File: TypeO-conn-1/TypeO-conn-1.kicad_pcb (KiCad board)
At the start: 2 copper layers, 5 parts, among them J1 USB_C_Receptacle_USB2.0, J2 , SW1 SW_DIP_x01

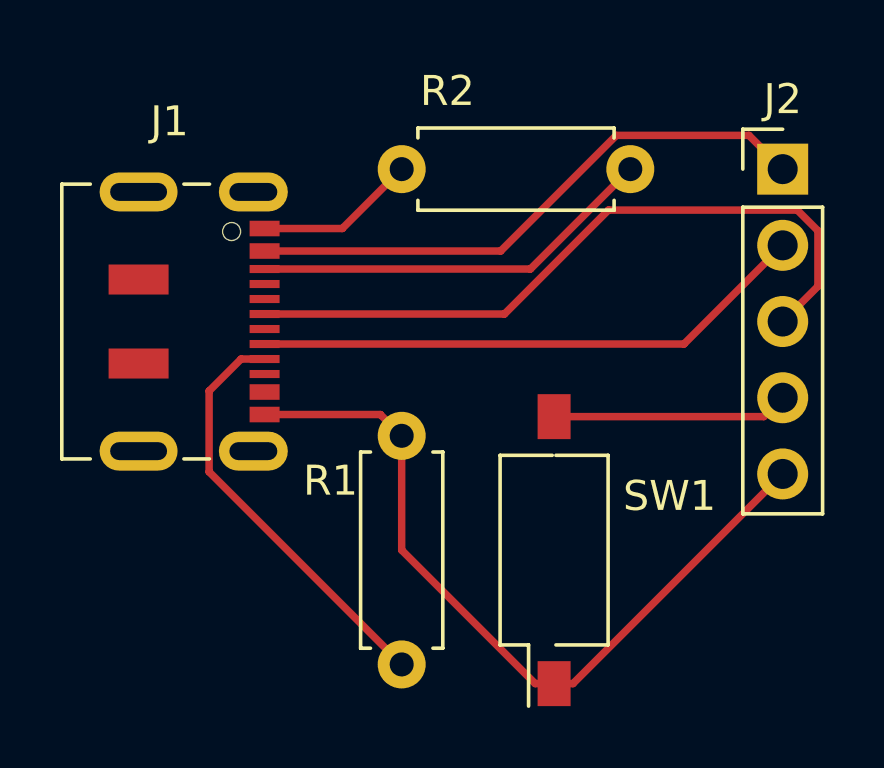
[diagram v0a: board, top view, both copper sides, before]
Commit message: Update PCB
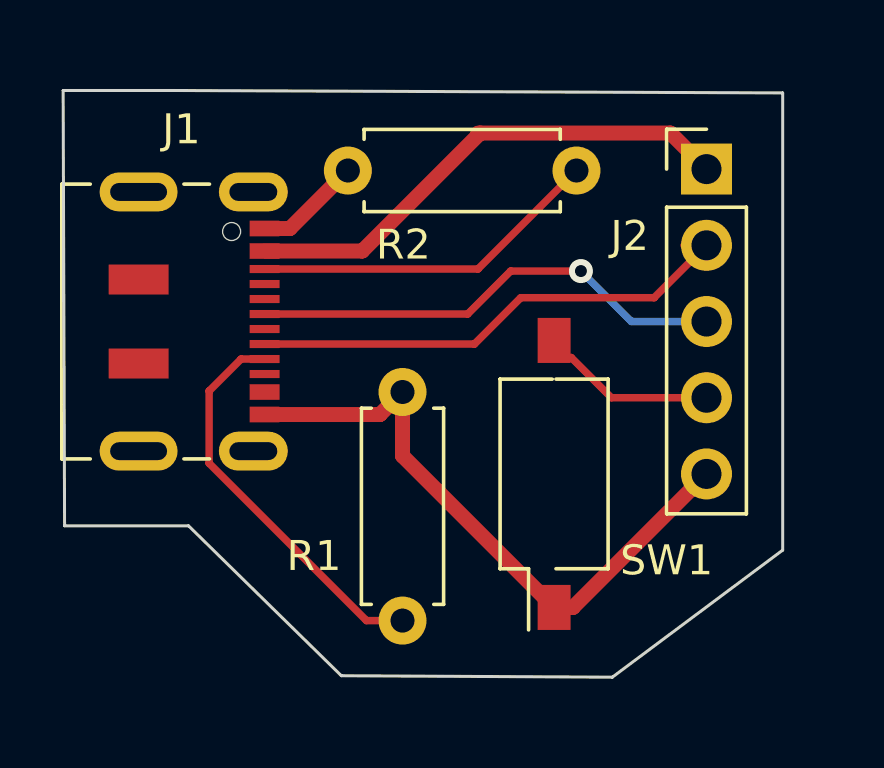
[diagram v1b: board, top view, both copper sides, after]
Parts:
- moved J2 2.54 mm to (124.5, 76.2)
- moved SW1 2.54 mm to (119.4, 86.4)
- moved R2 1.79 mm to (112.5, 76.2)
- moved R1 1.46 mm to (114.3, 83.6)
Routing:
- net Net-(J1-PadA6): track 23.7 -> 16.0 mm, vias 0 -> 1
- net Net-(J1-PadA1): track 31.5 -> 24.7 mm
- net Net-(J1-PadA4): track 19.3 -> 16.9 mm
- net Net-(SW1-Pad2): track 7.88 -> 5.64 mm
- net Net-(J1-PadA5): track 13.6 -> 11.8 mm
- net Net-(J1-PadA7): track 18.6 -> 16.8 mm
- net Net-(J1-PadB5): track 14.1 -> 13.3 mm
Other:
- board outline added: 24 x 19.6 mm
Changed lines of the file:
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@@
     (property "Sheetname" "")
     (attr smd)
-    (fp_text reference "J1" (at -6.670499 0.12134 180) (layer "F.SilkS")
+    (fp_text reference "J1" (at -6.404035 -0.274964 180) (layer "F.SilkS")
       (effects (font (size 1 1) (thickness 0.15)))
     )
@@
   )
   (footprint "Resistor_THT:R_Axial_DIN0207_L6.3mm_D2.5mm_P7.62mm_Horizontal" (layer "F.Cu")
-    (at 114.3 76.2)
+    (at 112.505976 76.246718)
     (descr "Resistor, Axial_DIN0207 series, Axial, Horizontal, pin pitch=7.62mm, 0.25W = 1/4W, length*diameter=6.3*2.5mm^2, http://cdn-reichelt.de/documents/datenblatt/B400/1_4W%23YAG.pdf")
     (tags "Resistor Axial_DIN0207 series Axial Horizontal pin pitch 7.62mm 0.25W = 1/4W length 6.3mm diameter 2.5mm")
@@
     (property "Sheetname" "")
     (attr through_hole)
-    (fp_text reference "R2" (at 1.522976 -2.602604) (layer "F.SilkS")
-      (effects (font (size 1 1) (thickness 0.15)))
-    )
-    (fp_text value "10K" (at 5.08 -2.54) (layer "F.Fab")
+    (fp_text reference "R2" (at 1.848743 2.473275) (layer "F.SilkS")
+      (effects (font (size 1 1) (thickness 0.15)))
+    )
+    (fp_text value "10K" (at 5.54862 2.617426) (layer "F.Fab")
       (effects (font (size 1 1) (thickness 0.15)))
     )
@@
   )
   (footprint "Connector_PinHeader_2.54mm:PinHeader_1x05_P2.54mm_Vertical" (layer "F.Cu")
-    (at 127 76.2)
+    (at 124.46 76.2)
     (descr "Through hole straight pin header, 1x05, 2.54mm pitch, single row")
     (tags "Through hole pin header THT 1x05 2.54mm single row")
@@
     (property "Sheetname" "")
     (attr through_hole)
-    (fp_text reference "J2" (at 0 -2.33) (layer "F.SilkS")
+    (fp_text reference "J2" (at -2.561376 2.231691) (layer "F.SilkS")
       (effects (font (size 1 1) (thickness 0.15)))
     )
@@
   )
   (footprint "Resistor_THT:R_Axial_DIN0207_L6.3mm_D2.5mm_P7.62mm_Horizontal" (layer "F.Cu")
-    (at 114.3 85.09 -90)
+    (at 114.327258 83.628569 -90)
     (descr "Resistor, Axial_DIN0207 series, Axial, Horizontal, pin pitch=7.62mm, 0.25W = 1/4W, length*diameter=6.3*2.5mm^2, http://cdn-reichelt.de/documents/datenblatt/B400/1_4W%23YAG.pdf")
     (tags "Resistor Axial_DIN0207 series Axial Horizontal pin pitch 7.62mm 0.25W = 1/4W length 6.3mm diameter 2.5mm")
@@
     (property "Sheetname" "")
     (attr through_hole)
-    (fp_text reference "R1" (at 1.4988 2.373258 180) (layer "F.SilkS")
-      (effects (font (size 1 1) (thickness 0.15)))
-    )
-    (fp_text value "10K" (at 4.719649 2.429764 90) (layer "F.Fab")
+    (fp_text reference "R1" (at 5.470301 2.951661 180) (layer "F.SilkS")
+      (effects (font (size 1 1) (thickness 0.15)))
+    )
+    (fp_text value "10K" (at 1.482121 2.375057 90) (layer "F.Fab")
       (effects (font (size 1 1) (thickness 0.15)))
     )
@@
   )
   (footprint "Button_Switch_SMD:SW_DIP_SPSTx01_Slide_Omron_A6S-110x_W8.9mm_P2.54mm" (layer "F.Cu")
-    (at 119.38 88.9 90)
+    (at 119.38 86.36 90)
     (descr "SMD 1x-dip-switch SPST Omron_A6S-110x, Slide, row spacing 8.9 mm (350 mils), body size  (see http://omronfs.omron.com/en_US/ecb/products/pdf/en-a6s.pdf)")
     (tags "SMD DIP Switch SPST Slide 8.9mm 350mil")
@@
     (property "Sheetname" "")
     (attr smd)
-    (fp_text reference "SW1" (at 1.802645 3.847967 180) (layer "F.SilkS")
+    (fp_text reference "SW1" (at -2.883021 3.75 180) (layer "F.SilkS")
       (effects (font (size 1 1) (thickness 0.15)))
     )
@@
     )
   )
-  (segment (start 114.3 88.9) (end 114.3 85.09) (width 0.25) (layer "F.Cu") (net 1))
-  (segment (start 127 86.36) (end 120.01 93.35) (width 0.25) (layer "F.Cu") (net 1))
-  (segment (start 113.59 84.38) (end 109.73 84.38) (width 0.25) (layer "F.Cu") (net 1))
-  (segment (start 114.3 85.09) (end 113.59 84.38) (width 0.25) (layer "F.Cu") (net 1))
-  (segment (start 114.3 76.2) (end 112.32 78.18) (width 0.25) (layer "F.Cu") (net 1))
-  (segment (start 118.75 93.35) (end 114.3 88.9) (width 0.25) (layer "F.Cu") (net 1))
-  (segment (start 112.32 78.18) (end 109.73 78.18) (width 0.25) (layer "F.Cu") (net 1))
-  (segment (start 119.38 93.35) (end 118.75 93.35) (width 0.25) (layer "F.Cu") (net 1))
-  (segment (start 120.01 93.35) (end 119.38 93.35) (width 0.25) (layer "F.Cu") (net 1))
-  (segment (start 121.454211 75.075489) (end 117.5997 78.93) (width 0.25) (layer "F.Cu") (net 2))
-  (segment (start 117.5997 78.93) (end 109.73 78.93) (width 0.25) (layer "F.Cu") (net 2))
-  (segment (start 127 76.2) (end 125.875489 75.075489) (width 0.25) (layer "F.Cu") (net 2))
-  (segment (start 125.875489 75.075489) (end 121.454211 75.075489) (width 0.25) (layer "F.Cu") (net 2))
-  (segment (start 121.92 76.2) (end 118.59 79.53) (width 0.25) (layer "F.Cu") (net 3))
-  (segment (start 118.59 79.53) (end 109.73 79.53) (width 0.25) (layer "F.Cu") (net 3))
+  (gr_line (start 127 73.66) (end 127 88.9) (layer "Edge.Cuts") (width 0.1))
+  (gr_line (start 127 88.9) (end 121.32202 93.135099) (layer "Edge.Cuts") (width 0.1))
+  (gr_line (start 112.288553 93.087049) (end 107.195216 88.089812) (layer "Edge.Cuts") (width 0.1))
+  (gr_line (start 103.062885 88.089812) (end 103.014836 73.578605) (layer "Edge.Cuts") (width 0.1))
+  (gr_line (start 107.195216 88.089812) (end 103.062885 88.089812) (layer "Edge.Cuts") (width 0.1))
+  (gr_line (start 121.32202 93.135099) (end 112.288553 93.087049) (layer "Edge.Cuts") (width 0.1))
+  (gr_line (start 103.014836 73.578605) (end 106.68 73.578605) (layer "Edge.Cuts") (width 0.1))
+  (gr_line (start 106.68 73.578605) (end 127 73.66) (layer "Edge.Cuts") (width 0.1))
+  (segment (start 114.327258 85.757258) (end 119.38 90.81) (width 0.5) (layer "F.Cu") (net 1))
+  (segment (start 113.575827 84.38) (end 114.327258 83.628569) (width 0.5) (layer "F.Cu") (net 1))
+  (segment (start 120.01 90.81) (end 124.46 86.36) (width 0.5) (layer "F.Cu") (net 1))
+  (segment (start 119.38 90.81) (end 120.01 90.81) (width 0.5) (layer "F.Cu") (net 1))
+  (segment (start 110.572694 78.18) (end 109.73 78.18) (width 0.5) (layer "F.Cu") (net 1))
+  (segment (start 114.327258 83.628569) (end 114.327258 85.757258) (width 0.5) (layer "F.Cu") (net 1))
+  (segment (start 109.73 84.38) (end 113.575827 84.38) (width 0.5) (layer "F.Cu") (net 1))
+  (segment (start 112.505976 76.246718) (end 110.572694 78.18) (width 0.5) (layer "F.Cu") (net 1))
+  (segment (start 116.918282 74.997207) (end 112.985489 78.93) (width 0.5) (layer "F.Cu") (net 2))
+  (segment (start 112.985489 78.93) (end 109.73 78.93) (width 0.5) (layer "F.Cu") (net 2))
+  (segment (start 123.257207 74.997207) (end 116.84 74.997207) (width 0.5) (layer "F.Cu") (net 2))
+  (segment (start 124.46 76.2) (end 123.257207 74.997207) (width 0.5) (layer "F.Cu") (net 2))
+  (segment (start 116.842694 79.53) (end 109.73 79.53) (width 0.25) (layer "F.Cu") (net 3))
+  (segment (start 120.125976 76.246718) (end 116.842694 79.53) (width 0.25) (layer "F.Cu") (net 3))
+  (segment (start 114.327258 91.248569) (end 113.12539 91.248569) (width 0.25) (layer "F.Cu") (net 5))
   (segment (start 107.88048 83.595498) (end 108.945978 82.53) (width 0.25) (layer "F.Cu") (net 5))
-  (segment (start 107.88048 86.29048) (end 107.88048 83.595498) (width 0.25) (layer "F.Cu") (net 5))
   (segment (start 108.945978 82.53) (end 109.73 82.53) (width 0.25) (layer "F.Cu") (net 5))
-  (segment (start 114.3 92.71) (end 107.88048 86.29048) (width 0.25) (layer "F.Cu") (net 5))
-  (segment (start 121.190229 77.565489) (end 127.486499 77.565489) (width 0.25) (layer "F.Cu") (net 10))
-  (segment (start 109.73 81.03) (end 117.725718 81.03) (width 0.25) (layer "F.Cu") (net 10))
-  (segment (start 128.174511 80.105489) (end 127 81.28) (width 0.25) (layer "F.Cu") (net 10))
-  (segment (start 117.725718 81.03) (end 121.190229 77.565489) (width 0.25) (layer "F.Cu") (net 10))
-  (segment (start 128.174511 78.253501) (end 128.174511 80.105489) (width 0.25) (layer "F.Cu") (net 10))
-  (segment (start 127.486499 77.565489) (end 128.174511 78.253501) (width 0.25) (layer "F.Cu") (net 10))
-  (segment (start 109.73 82.03) (end 123.71 82.03) (width 0.25) (layer "F.Cu") (net 11))
-  (segment (start 123.71 82.03) (end 127 78.74) (width 0.25) (layer "F.Cu") (net 11))
-  (segment (start 126.37 84.45) (end 127 83.82) (width 0.25) (layer "F.Cu") (net 12))
-  (segment (start 119.38 84.45) (end 126.37 84.45) (width 0.25) (layer "F.Cu") (net 12))
+  (segment (start 113.12539 91.248569) (end 107.88048 86.003659) (width 0.25) (layer "F.Cu") (net 5))
+  (segment (start 107.88048 86.003659) (end 107.88048 83.595498) (width 0.25) (layer "F.Cu") (net 5))
+  (segment (start 117.931641 79.597769) (end 120.273755 79.597769) (width 0.25) (layer "F.Cu") (net 10))
+  (segment (start 109.73 81.03) (end 116.49941 81.03) (width 0.25) (layer "F.Cu") (net 10))
+  (segment (start 116.49941 81.03) (end 117.931641 79.597769) (width 0.25) (layer "F.Cu") (net 10))
+  (via (at 120.273755 79.597769) (size 0.8) (drill 0.4) (layers "F.Cu" "B.Cu") (net 10))
+  (segment (start 121.955986 81.28) (end 120.273755 79.597769) (width 0.25) (layer "B.Cu") (net 10))
+  (segment (start 124.46 81.28) (end 121.955986 81.28) (width 0.25) (layer "B.Cu") (net 10))
+  (segment (start 123.71 78.74) (end 124.46 78.74) (width 0.25) (layer "F.Cu") (net 11))
+  (segment (start 118.269603 80.486115) (end 122.713885 80.486115) (width 0.25) (layer "F.Cu") (net 11))
+  (segment (start 116.725718 82.03) (end 118.269603 80.486115) (width 0.25) (layer "F.Cu") (net 11))
+  (segment (start 109.73 82.03) (end 116.725718 82.03) (width 0.25) (layer "F.Cu") (net 11))
+  (segment (start 122.713885 80.486115) (end 124.46 78.74) (width 0.25) (layer "F.Cu") (net 11))
+  (segment (start 119.38 82.47952) (end 119.94952 82.47952) (width 0.25) (layer "F.Cu") (net 12))
+  (segment (start 121.29 83.82) (end 124.46 83.82) (width 0.25) (layer "F.Cu") (net 12))
+  (segment (start 119.94952 82.47952) (end 121.29 83.82) (width 0.25) (layer "F.Cu") (net 12))
 )
